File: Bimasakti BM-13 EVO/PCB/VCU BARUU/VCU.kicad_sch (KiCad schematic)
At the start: 31 parts, among them J1 6437288-3, U1 Teensy4.1, U11 ADS1115IDGS, U2 SN65HVD230, U3 SN65HVD230, U4 ADS1115IDGS, U5 SN65HVD230

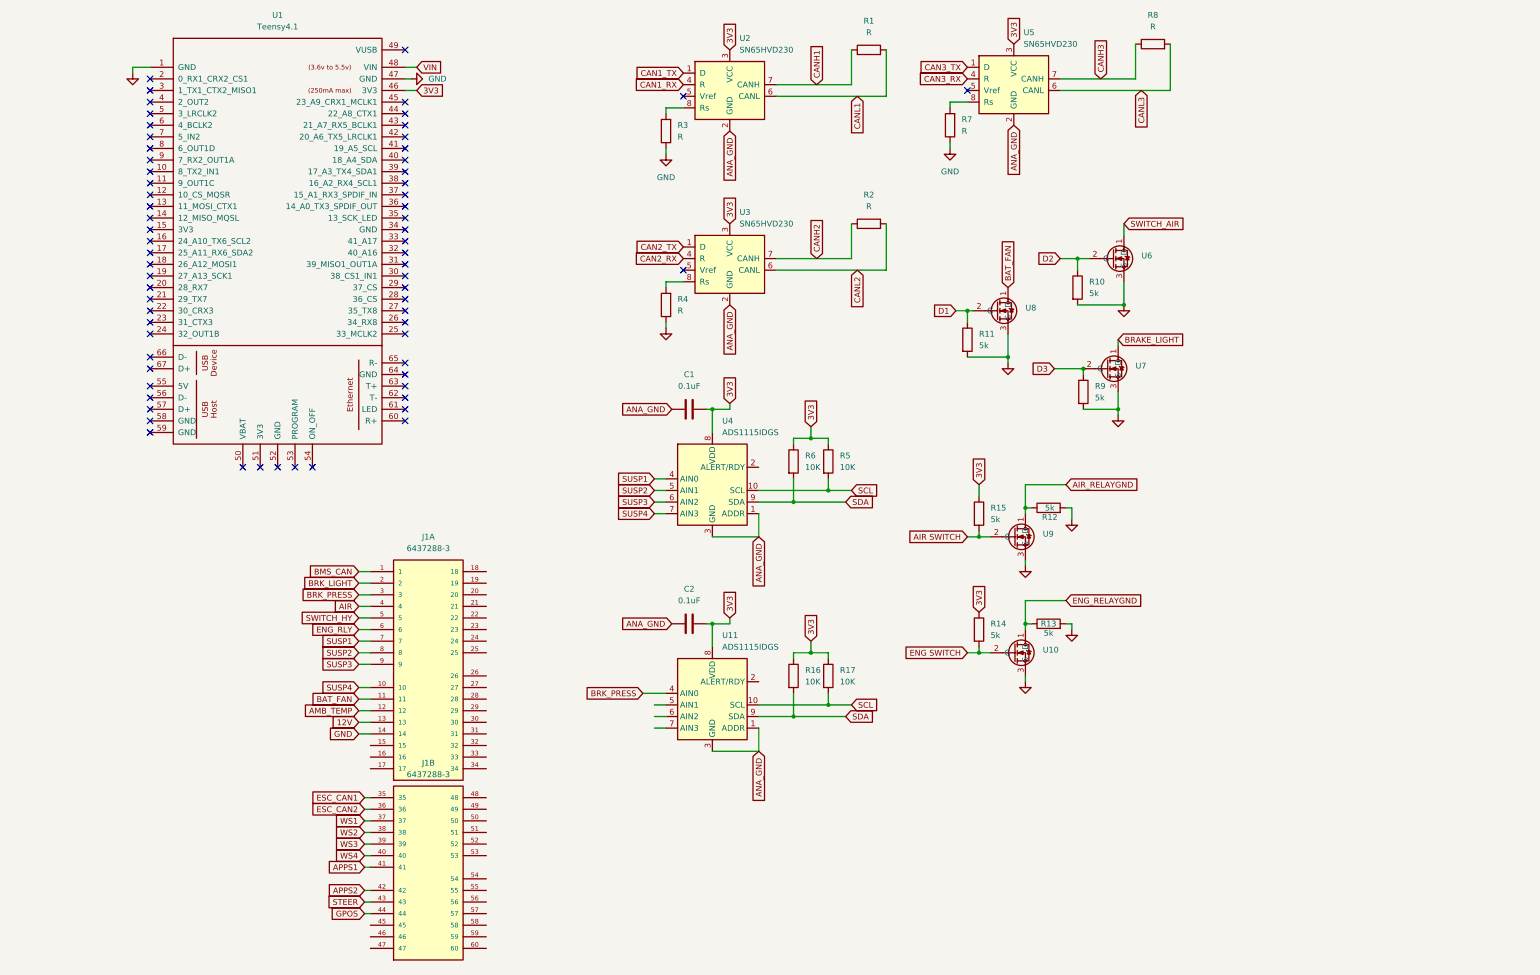
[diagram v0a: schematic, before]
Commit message: Aku Telemetry
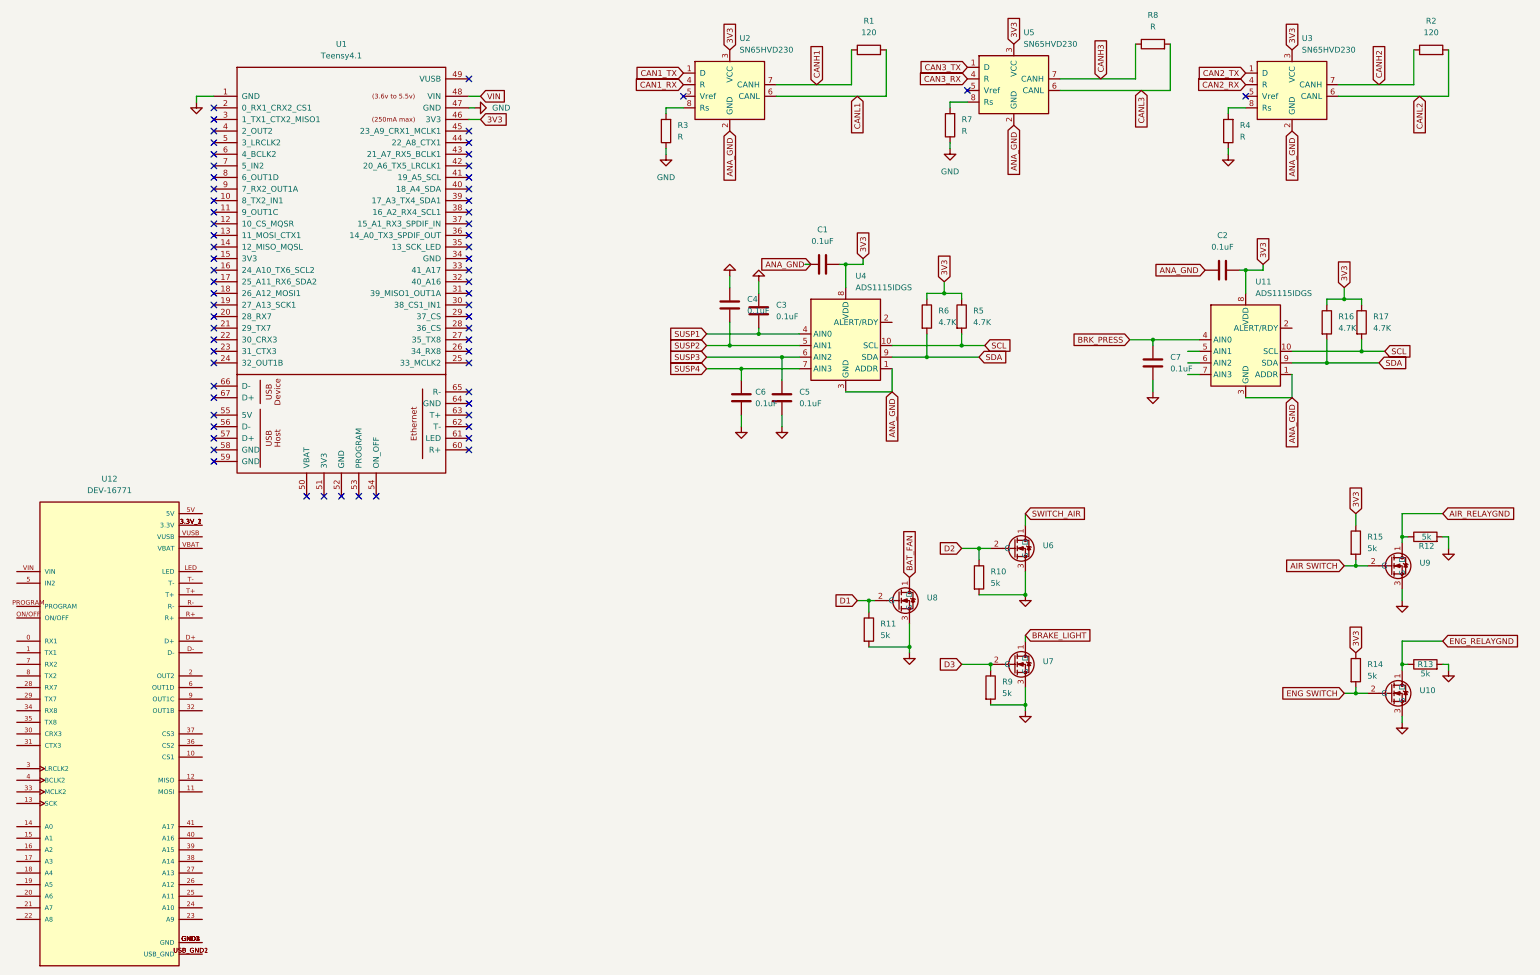
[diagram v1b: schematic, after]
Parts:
- removed J1: 6437288-3, 0_VCU_CONNECTOR_TE_6437288-3:VCU_CONNECTOR_TE_6437288-3, symbol 0_VCU_connector_6437288-3:6437288-3
- added C3, C4, C5, C6, C7: 0.1uF, Capacitor_SMD:C_0603_1608Metric, symbol Device:C
- added U12: DEV-16771, Teensy:Teensy41, symbol DEV-16771:DEV-16771
- R1, R2: value R -> 120
- R16, R17, R5, R6: value 10K -> 4.7K
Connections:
- net BRK_PRESS: now also C7.2
- net GND: now also C3.2, C4.2, C5.1, C6.1, C7.1
- net SUSP1: now also C3.1
- net SUSP2: now also C4.1
- net SUSP3: now also C5.2
- net SUSP4: now also C6.2
- new net: U12.3.3V_1 (3.3V), U12.3.3V_2 (3.3V), U12.3.3V_3 (3.3V)
- new net: U12.GND1 (GND), U12.GND2 (GND), U12.GND3 (GND), U12.GND4 (GND), U12.GND5 (GND)
- new net: U12.USB_GND1 (USB_GND), U12.USB_GND2 (USB_GND)
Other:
- moved on the sheet: C1, C2, R10, R11, R12, R13, R14, R15, R16, R17, R2, R4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
